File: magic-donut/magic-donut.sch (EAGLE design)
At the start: 46 parts

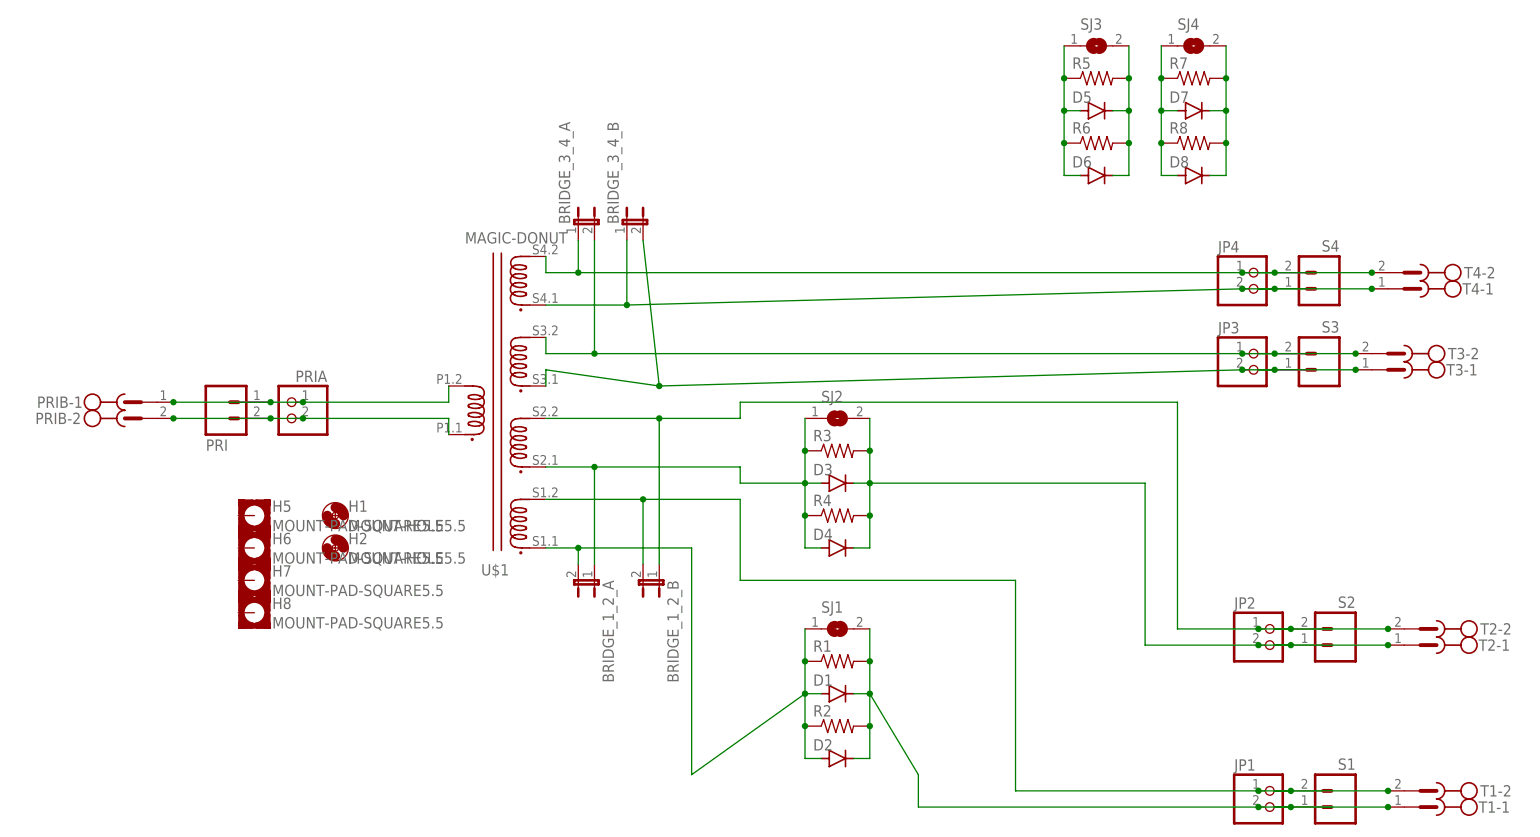
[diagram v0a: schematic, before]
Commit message: Work with @eranrund
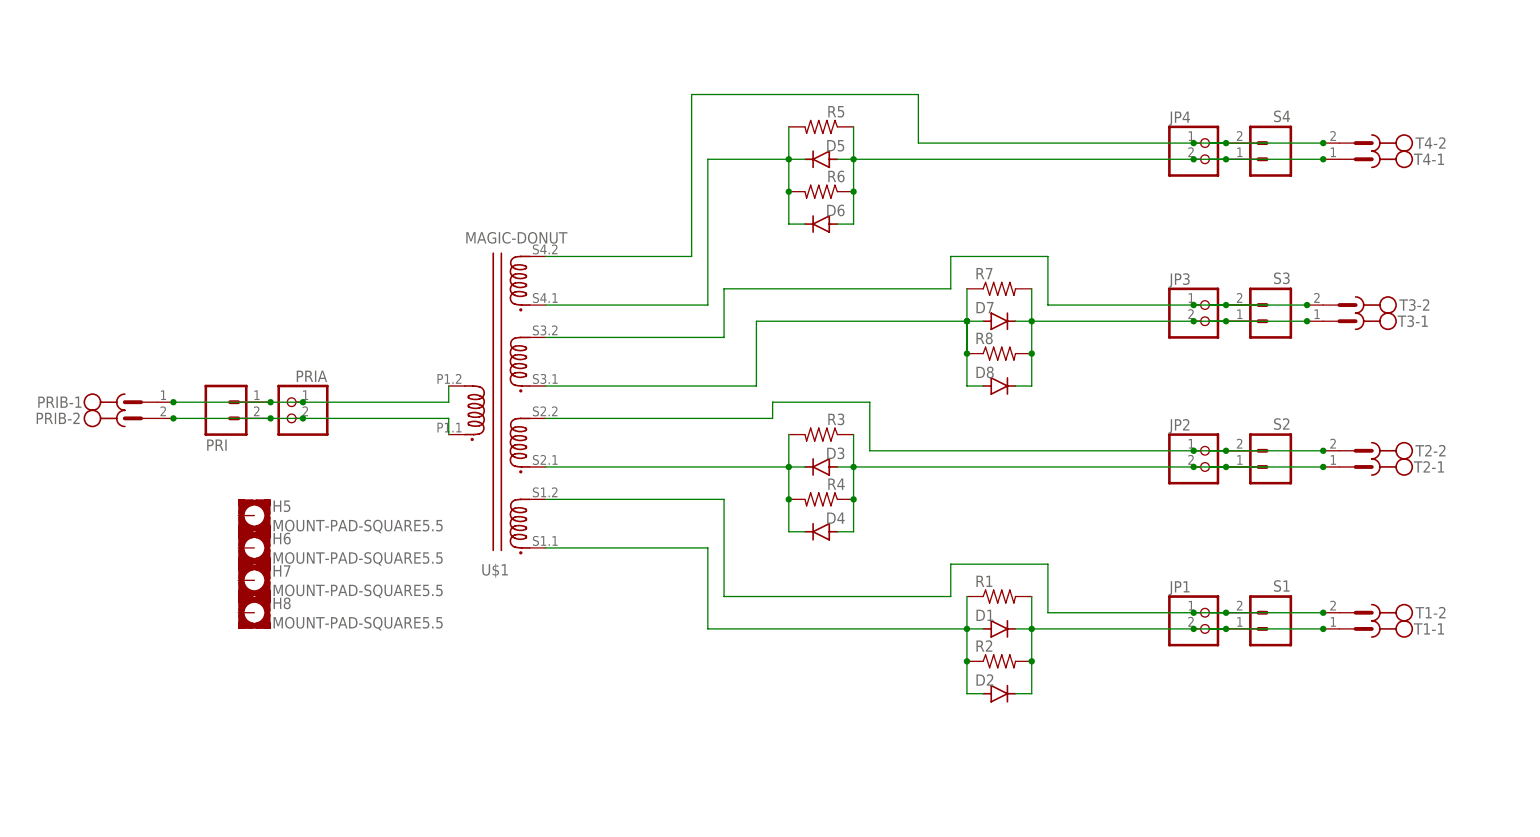
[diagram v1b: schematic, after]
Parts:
- removed BRIDGE_1_2_A, BRIDGE_1_2_B, BRIDGE_3_4_A, BRIDGE_3_4_B: (no value), jumper:JP1E
- removed H1, H2: MOUNT-HOLE5.5, holes:MOUNT-HOLE5.5
- removed SJ1, SJ2, SJ3, SJ4: (no value), jumper:SJ
- R2, R4, R6, R8: device rcl:R-US_0207/2V -> rcl:R-US_0207/7
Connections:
- removed net N$1: BRIDGE_1_2_A.2, D1.A, D2.A, R1.1, R2.1, SJ1.1, U$1.S1.1
- removed net N$13: D1.C, D2.C, JP1.2, R1.2, R2.2, S1.1, SJ1.2, T1-1.SK
- removed net N$16: D3.C, D4.C, JP2.2, R3.2, R4.2, S2.1, SJ2.2, T2-1.SK
- removed net N$18: D5.C, D6.C, R5.2, R6.2, SJ3.2
- removed net N$19: D7.A, D8.A, R7.1, R8.1, SJ4.1
- removed net N$2: BRIDGE_1_2_B.2, JP1.1, S1.2, T1-2.SK, U$1.S1.2
- removed net N$3: BRIDGE_3_4_A.1, JP4.1, S4.2, T4-2.SK, U$1.S4.2
- removed net N$7: BRIDGE_1_2_B.1, JP2.1, S2.2, T2-2.SK, U$1.S2.2
- new net N$21: JP2.1, S2.2, T2-2.SK, U$1.S2.2
- new net N$22: D3.C, D4.C, R3.2, R4.2, U$1.S2.1
- new net N$23: JP1.1, S1.2, T1-2.SK, U$1.S1.2
- new net N$26: D1.C, D2.C, JP1.2, R1.2, R2.2, S1.1, T1-1.SK
- new net N$9: JP4.1, S4.2, T4-2.SK, U$1.S4.2
- new net S1-1: D1.A, D2.A, R1.1, R2.1, U$1.S1.1
- net N$17: now also JP4.2, S4.1, T4-1.SK; no longer SJ3.1
- net N$20: now also JP3.2, S3.1, T3-1.SK; no longer SJ4.2
- net N$4: now also D5.C, D6.C, R5.2, R6.2; no longer BRIDGE_3_4_B.1, JP4.2, S4.1, T4-1.SK
- net N$5: no longer BRIDGE_3_4_A.2
- net N$6: now also D7.A, D8.A, R7.1, R8.1; no longer BRIDGE_3_4_B.2, JP3.2, S3.1, T3-1.SK
- net N$8: now also JP2.2, S2.1, T2-1.SK; no longer BRIDGE_1_2_A.1, SJ2.1, U$1.S2.1
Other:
- moved on the sheet: D1, D2, D3, D4, D5, D6, D7, D8, JP1, JP2, JP3, JP4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
